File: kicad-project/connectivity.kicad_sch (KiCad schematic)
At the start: 9 parts

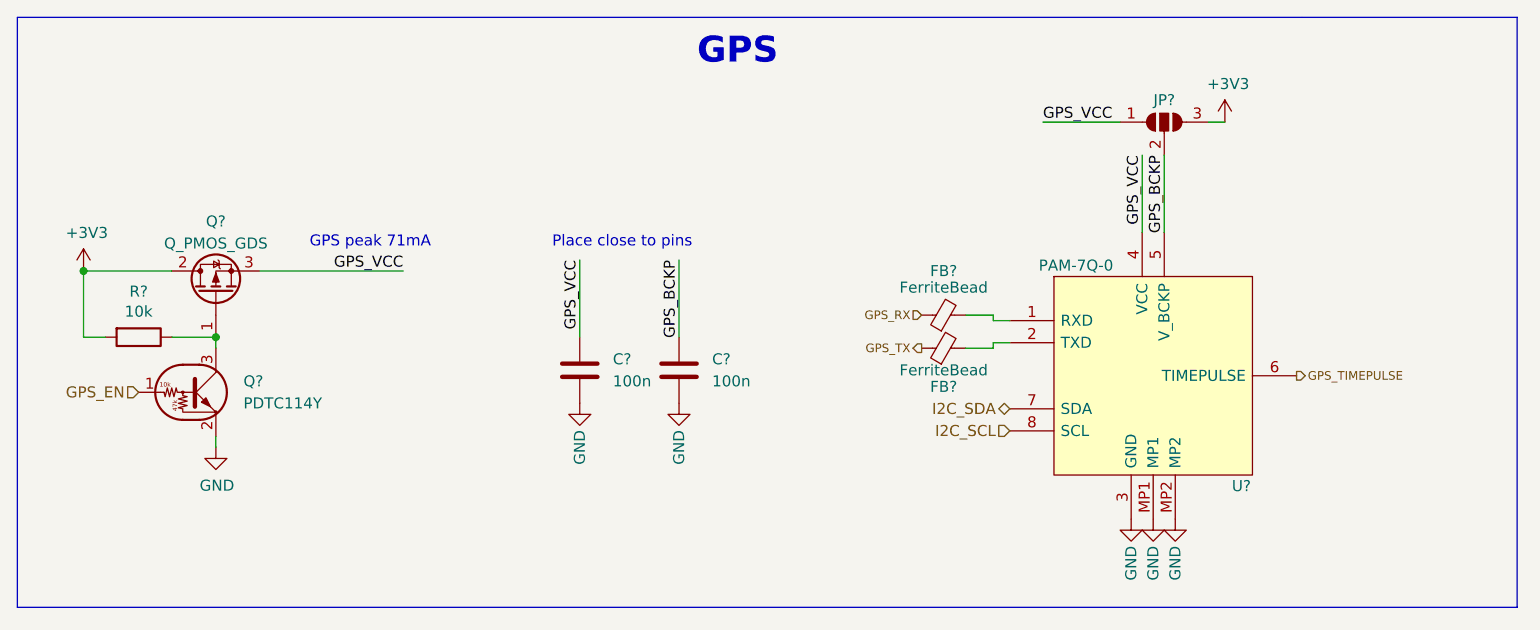
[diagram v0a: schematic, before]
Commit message: hw: schematic updates
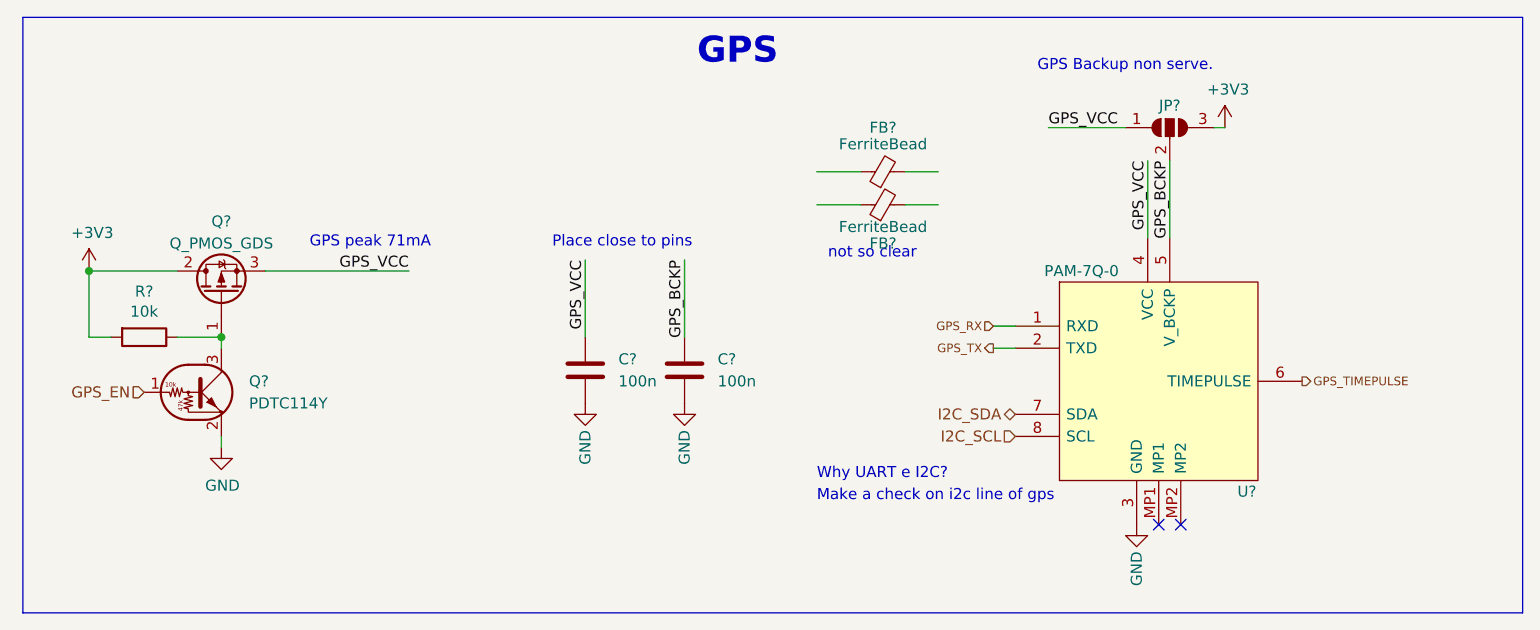
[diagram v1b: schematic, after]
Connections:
- net GND: no longer U?.MP1, U?.MP2
- net GPS_RX: now also U?.1 (RXD); no longer FB?.1
- net GPS_TX: now also U?.2 (TXD); no longer FB?.1
- net at FB?.2: no longer U?.1 (RXD)
- net at FB?.2: no longer U?.2 (TXD)
- no-connect marks 0 -> 2
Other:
- note added: "GPS Backup non serve."
- note added: "Make a check on i2c line of gps"
- note added: "Why UART e I2C?"
- note added: "not so clear"
- moved on the sheet: C?, FB?, JP?, Q?, R?, U?
